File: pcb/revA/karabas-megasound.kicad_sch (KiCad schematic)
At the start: 2 parts

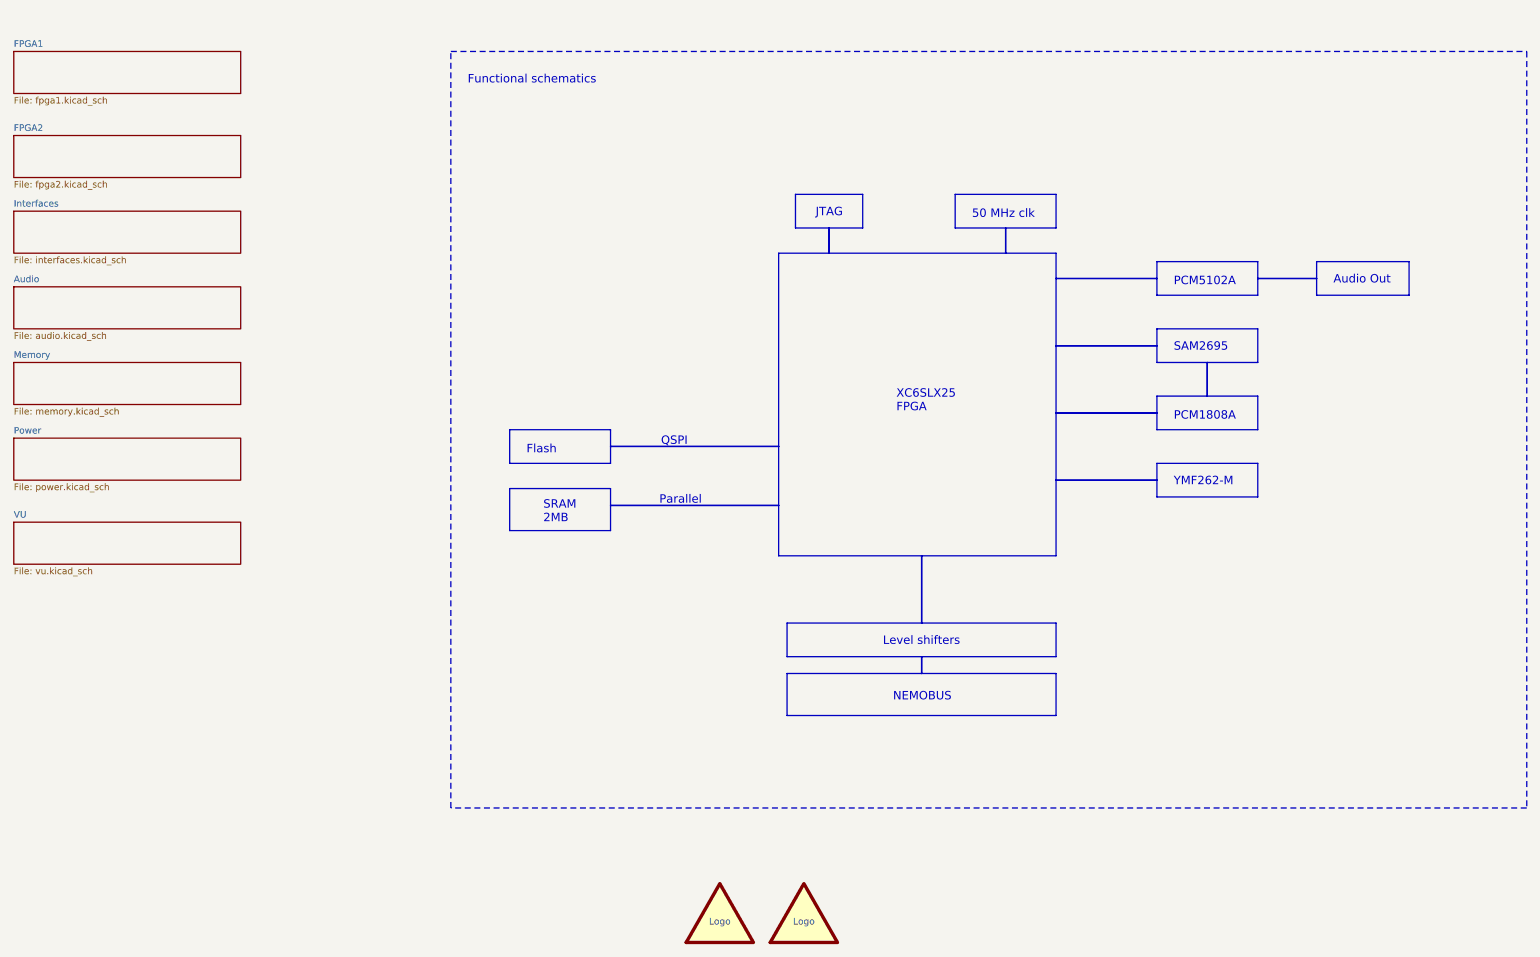
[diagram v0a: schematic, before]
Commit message: Initial firmware
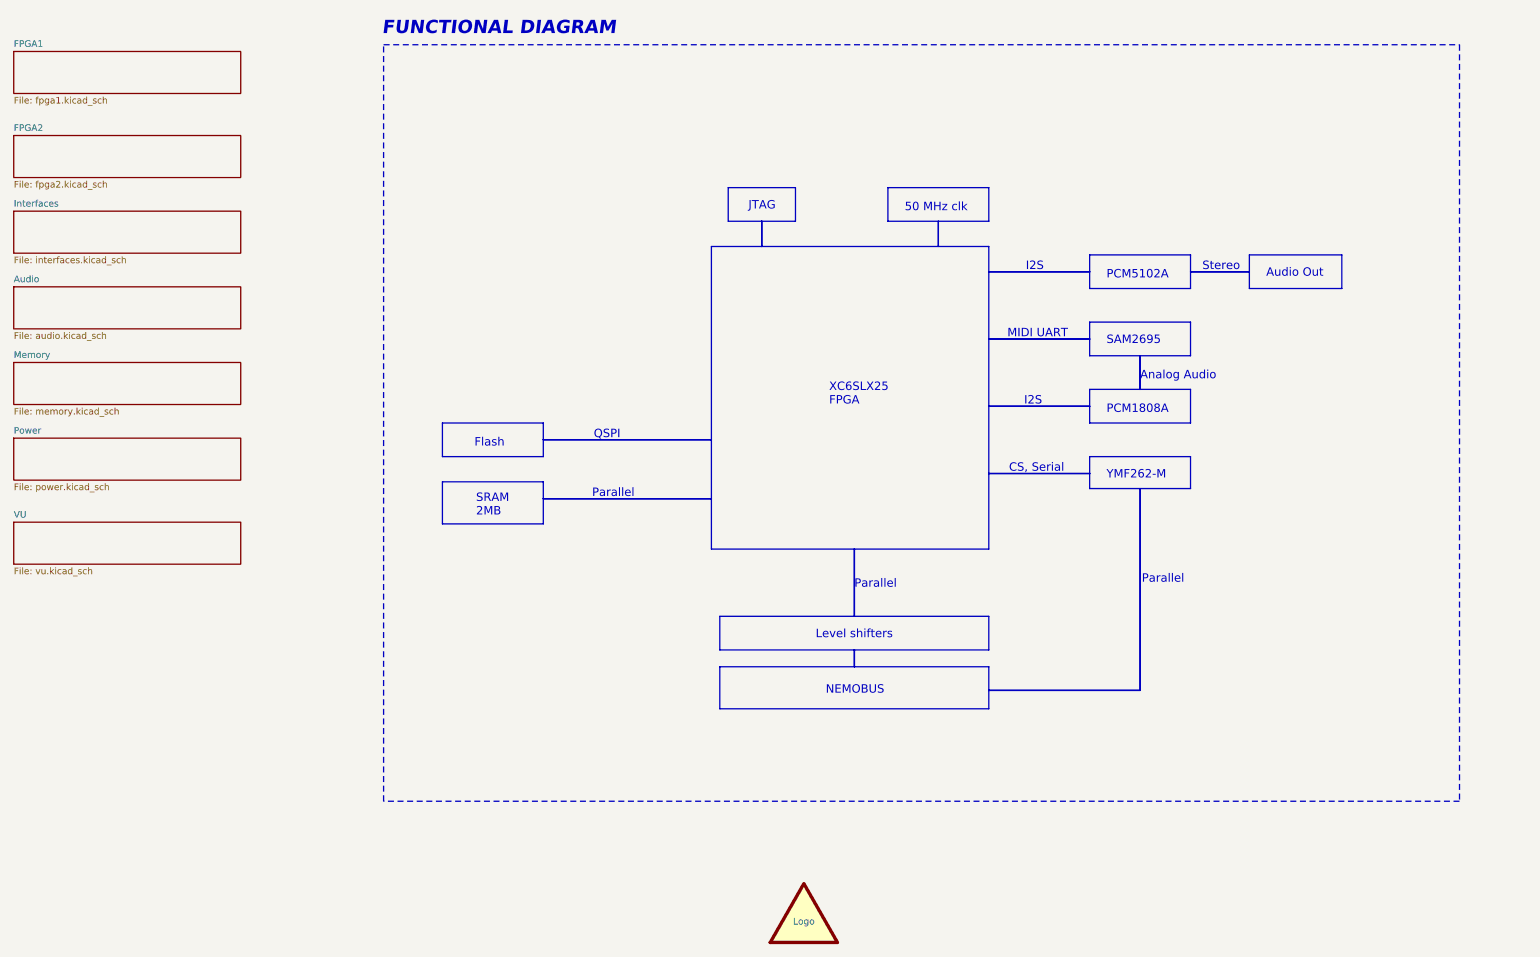
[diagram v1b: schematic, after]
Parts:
- removed LOGO1: graphic, footprints:opl3, symbol my:logo
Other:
- note added: "Analog Audio"
- note added: "CS, Serial"
- note added: "FUNCTIONAL DIAGRAM"
- note added: "I2S"
- note added: "MIDI UART"
- note added: "Stereo"
- note removed: "Functional schematics"
- title: karabas-Megasound -> Karabas-MegaBuzz
